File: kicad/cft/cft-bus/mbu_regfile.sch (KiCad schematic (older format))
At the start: 21 parts, among them J1 Conn_02x07_Counter_Clockwise, J2 Conn_02x07_Counter_Clockwise, U11 74HC670, U12 74AC541, U13 74LVC2G157, U14 74HC670, U15 74HC670, U9 74HC670

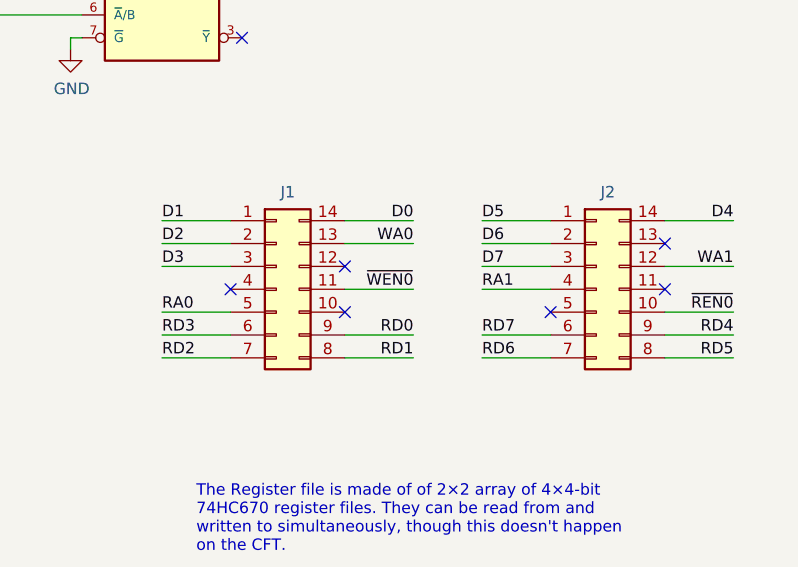
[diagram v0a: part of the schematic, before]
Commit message: Routing BUS board.
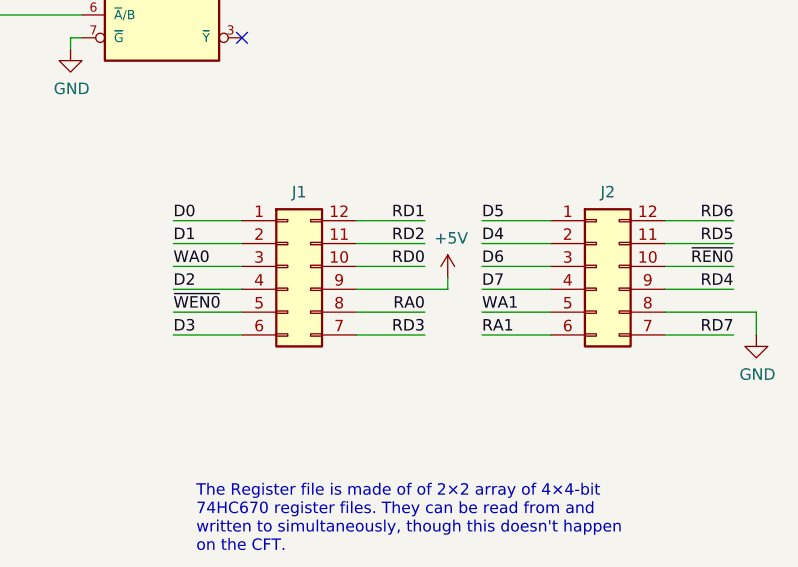
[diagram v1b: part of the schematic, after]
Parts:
- removed J1, J2: Conn_02x07_Counter_Clockwise, Connector_PinHeader_2.54mm:PinHeader_2x07_P2.54mm_Vertical, symbol Connector_Generic:Conn_02x07_Counter_Clockwise
- added J1, J2: Conn_02x06_Counter_Clockwise, Connector_PinHeader_2.54mm:PinHeader_2x06_P2.54mm_Vertical, symbol Connector_Generic:Conn_02x06_Counter_Clockwise
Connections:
- net +5V: now also J1.9 (Pin_9)
- net D0: now also J1.1 (Pin_1)
- net D1: now also J1.2 (Pin_2)
- net D2: now also J1.4 (Pin_4)
- net D3: now also J1.6 (Pin_6)
- net D4: now also J2.2 (Pin_2)
- net D5: now also J2.1 (Pin_1)
- net D6: now also J2.3 (Pin_3)
- net D7: now also J2.4 (Pin_4)
- net GND: now also J2.8 (Pin_8)
- net RA0: now also J1.8 (Pin_8)
- net RA1: now also J2.6 (Pin_6)
- net RD0: now also J1.10 (Pin_10)
- net RD1: now also J1.12 (Pin_12)
- net RD2: now also J1.11 (Pin_11)
- net RD3: now also J1.7 (Pin_7)
- net RD4: now also J2.9 (Pin_9)
- net RD5: now also J2.11 (Pin_11)
- net RD6: now also J2.12 (Pin_12)
- net RD7: now also J2.7 (Pin_7)
- net WA0: now also J1.3 (Pin_3)
- net WA1: now also J2.5 (Pin_5)
- net ~REN0: now also J2.10 (Pin_10)
- net ~WEN0: now also J1.5 (Pin_5)
- no-connect marks 8 -> 2
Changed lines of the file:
@@
 The Register file is made of of 2×2 array of 4×4-bit\n74HC670 register files. They can be read from and\nwritten to simultaneously, though this doesn't happen\non the CFT.\n\nA buffer allows the output of the register file to be\ntri-stated. Pull-down resistors and a multiplexer\nallow the register files to be disabled until needed.\n\nIn that case, AEXT will be hardwired to either &00\nor &80, depending on the state of the RAM/ROM\nswitch on the front panel.
 NoConn ~ 8350 3450
-$Comp
-L Connector_Generic:Conn_02x07_Counter_Clockwise J1
-U 1 1 6026A398
-P 8500 4550
-F 0 "J1" H 8550 4975 50  0000 C CNN
-F 1 "Conn_02x07_Counter_Clockwise" H 8550 4976 50  0001 C CNN
-F 2 "Connector_PinHeader_2.54mm:PinHeader_2x07_P2.54mm_Vertical" H 8500 4550 50  0001 C CNN
-F 3 "~" H 8500 4550 50  0001 C CNN
-	1    8500 4550
-	1    0    0    -1
-$EndComp
 Wire Wire Line
-	8300 4250 8000 4250
+	9400 4650 9700 4650
 Wire Wire Line
-	8300 4350 8000 4350
+	10500 4450 10200 4450
 Wire Wire Line
-	8300 4450 8000 4450
+	9700 4250 9400 4250
 Wire Wire Line
 	9700 4550 9400 4550
 Wire Wire Line
-	8300 4650 8000 4650
+	10200 4750 10500 4750
 Wire Wire Line
-	8300 4750 8000 4750
+	9400 4350 9700 4350
 Wire Wire Line
-	8300 4850 8000 4850
+	10500 4550 10200 4550
 Wire Wire Line
-	9100 4250 8800 4250
-Wire Wire Line
-	9100 4350 8800 4350
-Wire Wire Line
-	10500 4450 10200 4450
-Wire Wire Line
-	9100 4550 8800 4550
-Wire Wire Line
-	10500 4650 10200 4650
-Wire Wire Line
-	9100 4750 8800 4750
-Wire Wire Line
-	9100 4850 8800 4850
-$Comp
-L Connector_Generic:Conn_02x07_Counter_Clockwise J2
-U 1 1 602A65DB
-P 9900 4550
-F 0 "J2" H 9950 4975 50  0000 C CNN
-F 1 "Conn_02x07_Counter_Clockwise" H 9950 4976 50  0001 C CNN
-F 2 "Connector_PinHeader_2.54mm:PinHeader_2x07_P2.54mm_Vertical" H 9900 4550 50  0001 C CNN
-F 3 "~" H 9900 4550 50  0001 C CNN
-	1    9900 4550
-	1    0    0    -1
-$EndComp
-Wire Wire Line
-	9700 4250 9400 4250
-Wire Wire Line
-	9700 4350 9400 4350
+	10500 4350 10200 4350
+Text Label 9400 4350 0    50   ~ 0
+D4
+Text Label 9400 4250 0    50   ~ 0
+D5
+Text Label 9400 4450 0    50   ~ 0
+D6
+Text Label 9400 4550 0    50   ~ 0
+D7
+Text Label 9400 4650 0    50   ~ 0
+WA1
+Text Label 9400 4750 0    50   ~ 0
+RA1
+Text Label 10500 4450 2    50   ~ 0
+~REN0
+Text Label 10500 4750 2    50   ~ 0
+RD7
+Text Label 10500 4550 2    50   ~ 0
+RD4
+Text Label 10500 4350 2    50   ~ 0
+RD5
 Wire Wire Line
 	9700 4450 9400 4450
 Wire Wire Line
 	9700 4750 9400 4750
+Text Label 10500 4250 2    50   ~ 0
+RD6
 Wire Wire Line
-	9700 4850 9400 4850
+	10200 4250 10500 4250
+Text Label 9150 4350 2    50   ~ 0
+RD2
+Text Label 8050 4550 0    50   ~ 0
+D2
+Text Label 8050 4350 0    50   ~ 0
+D1
 Wire Wire Line
-	10500 4250 10200 4250
+	8850 4350 9150 4350
 Wire Wire Line
-	10500 4750 10200 4750
+	8350 4550 8050 4550
 Wire Wire Line
-	10500 4850 10200 4850
-Text Label 8000 4250 0    50   ~ 0
-D1
-Text Label 9100 4250 2    50   ~ 0
+	8350 4350 8050 4350
+Text Label 9150 4250 2    50   ~ 0
+RD1
+Text Label 8050 4650 0    50   ~ 0
+~WEN0
+Text Label 8050 4450 0    50   ~ 0
+WA0
+Text Label 8050 4250 0    50   ~ 0
 D0
-Text Label 8000 4350 0    50   ~ 0
-D2
-Text Label 8000 4450 0    50   ~ 0
+Wire Wire Line
+	9150 4250 8850 4250
+Wire Wire Line
+	8050 4650 8350 4650
+Wire Wire Line
+	8050 4450 8350 4450
+Wire Wire Line
+	8050 4250 8350 4250
+Wire Wire Line
+	8350 4750 8050 4750
+Wire Wire Line
+	8850 4650 9150 4650
+Text Label 8050 4750 0    50   ~ 0
 D3
-Text Label 10500 4250 2    50   ~ 0
-D4
-Text Label 9400 4250 0    50   ~ 0
-D5
-Text Label 9400 4350 0    50   ~ 0
-D6
-Text Label 9400 4450 0    50   ~ 0
-D7
-Text Label 9100 4350 2    50   ~ 0
-WA0
-Text Label 10500 4450 2    50   ~ 0
-WA1
-Text Label 9400 4550 0    50   ~ 0
-RA1
-Text Label 8000 4650 0    50   ~ 0
+Text Label 9150 4650 2    50   ~ 0
 RA0
-Text Label 8000 4750 0    50   ~ 0
+Wire Wire Line
+	8850 4750 9150 4750
+Text Label 9150 4750 2    50   ~ 0
 RD3
-Text Label 8000 4850 0    50   ~ 0
-RD2
-Text Label 9100 4550 2    50   ~ 0
-~WEN0
-Text Label 10500 4650 2    50   ~ 0
-~REN0
-Text Label 9100 4750 2    50   ~ 0
+Text Label 9150 4450 2    50   ~ 0
 RD0
-Text Label 9100 4850 2    50   ~ 0
-RD1
-Text Label 9400 4750 0    50   ~ 0
-RD7
-Text Label 9400 4850 0    50   ~ 0
-RD6
-Text Label 10500 4750 2    50   ~ 0
-RD4
-Text Label 10500 4850 2    50   ~ 0
-RD5
-NoConn ~ 8800 4450
-NoConn ~ 8300 4550
-NoConn ~ 10200 4350
-NoConn ~ 10200 4550
-NoConn ~ 8800 4650
-NoConn ~ 9700 4650
+Wire Wire Line
+	9150 4450 8850 4450
+$Comp
+L Connector_Generic:Conn_02x06_Counter_Clockwise J1
+U 1 1 60DE7914
+P 8550 4450
+F 0 "J1" H 8600 4775 50  0000 C CNN
+F 1 "Conn_02x06_Counter_Clockwise" H 8600 4776 50  0001 C CNN
+F 2 "Connector_PinHeader_2.54mm:PinHeader_2x06_P2.54mm_Vertical" H 8550 4450 50  0001 C CNN
+F 3 "~" H 8550 4450 50  0001 C CNN
+	1    8550 4450
+	1    0    0    -1
+$EndComp
+$Comp
+L Connector_Generic:Conn_02x06_Counter_Clockwise J2
+U 1 1 60E5FDEB
+P 9900 4450
+F 0 "J2" H 9950 4775 50  0000 C CNN
+F 1 "Conn_02x06_Counter_Clockwise" H 9950 4776 50  0001 C CNN
+F 2 "Connector_PinHeader_2.54mm:PinHeader_2x06_P2.54mm_Vertical" H 9900 4450 50  0001 C CNN
+F 3 "~" H 9900 4450 50  0001 C CNN
+	1    9900 4450
+	1    0    0    -1
+$EndComp
+Wire Wire Line
+	10200 4650 10600 4650
+Wire Wire Line
+	10600 4650 10600 4750
+$Comp
+L power:GND #PWR0160
+U 1 1 60E9A285
+P 10600 4750
+F 0 "#PWR0160" H 10600 4500 50  0001 C CNN
+F 1 "GND" H 10605 4577 50  0000 C CNN
+F 2 "" H 10600 4750 50  0001 C CNN
+F 3 "" H 10600 4750 50  0001 C CNN
+	1    10600 4750
+	1    0    0    -1
+$EndComp
+Wire Wire Line
+	8850 4550 9250 4550
+Wire Wire Line
+	9250 4550 9250 4500
 Wire Bus Line
 	6750 1250 6750 3350
 Wire Bus Line
 	4250 1250 4250 3350
+$Comp
+L power:+5V #PWR0161
+U 1 1 60EA4931
+P 9250 4500
+F 0 "#PWR0161" H 9250 4350 50  0001 C CNN
+F 1 "+5V" H 9265 4673 50  0000 C CNN
+F 2 "" H 9250 4500 50  0001 C CNN
+F 3 "" H 9250 4500 50  0001 C CNN
+	1    9250 4500
+	1    0    0    -1
+$EndComp
 $EndSCHEMATC
